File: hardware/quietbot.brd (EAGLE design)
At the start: 100 x 80 mm, 9 parts, among them IC2 REG1117

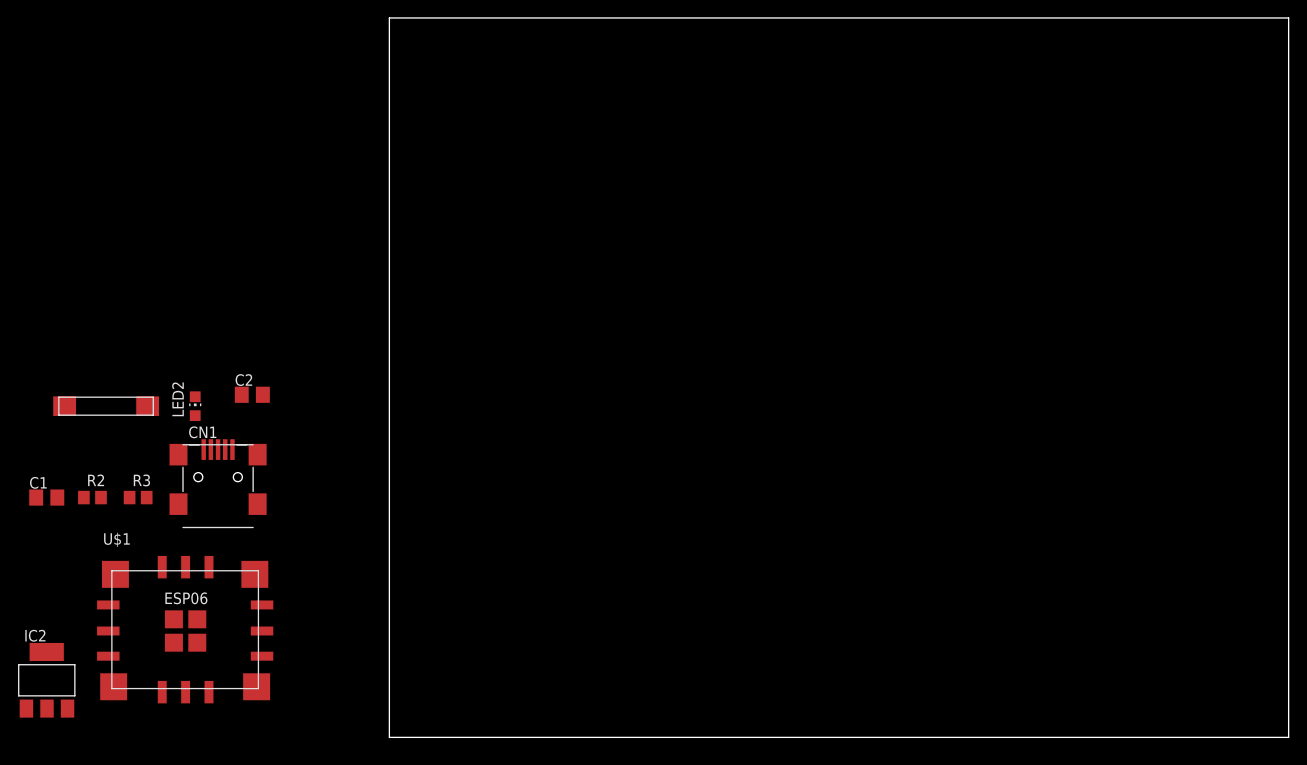
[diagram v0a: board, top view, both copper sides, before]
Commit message: board design
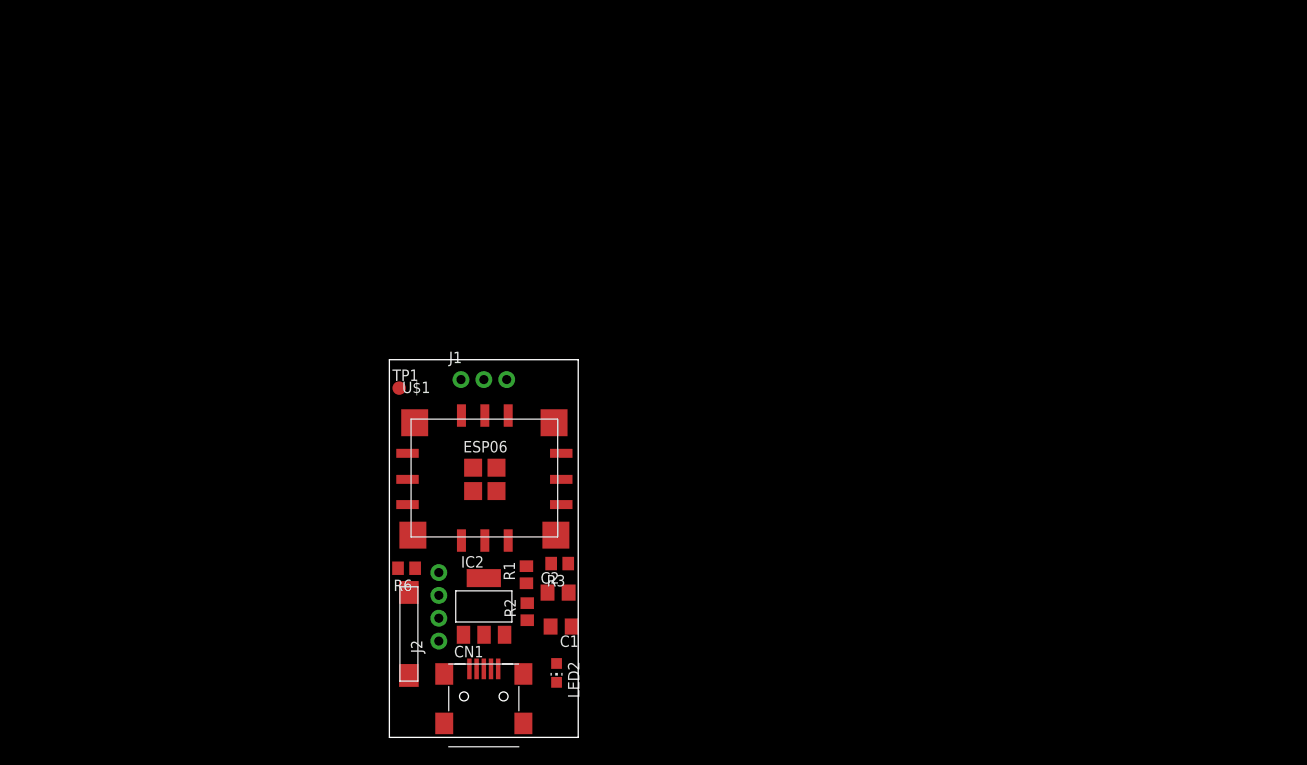
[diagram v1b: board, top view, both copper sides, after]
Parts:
- added J1: (no value), SparkFun-Connectors:1X03_NO_SILK
- added J2: (no value), SparkFun-Connectors:1X04_NO_SILK_ALL_ROUND
- added R1, R6: 10K, resistor:R0805
- added TP1: TPTP15R, testpad:TP15R
- moved C1 59.0 mm to (19.1, 12.3), turned to 180 degrees
- moved R2 50.0 mm to (15.3, 14.0), turned to 90 degrees
- moved LED2 49.9 mm to (18.6, 7.17), turned to 180 degrees
- moved IC2 49.3 mm to (10.5, 14.6)
- moved R3 47.5 mm to (18.9, 19.3), turned to 180 degrees
- moved U$2 42.5 mm to (2.17, 11.2), turned to 90 degrees
- moved C2 40.5 mm to (18.8, 16.1)
- moved CN1 38.3 mm to (10.5, 3.56)
- moved U$1 37.3 mm to (10.4, 28.3)
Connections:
- new net N$4: R6.2, TP1.TP, U$1.GPIO0
- new net N$5: R1.2, U$1.CH_PD
- new net RX: J2.2, U$1.RX
- new net SIG_PIXEL: J1.2, U$1.GPIO2
- new net TX: J2.3, U$1.TX
- net +3V3: now also J2.1, R1.1, R6.1; no longer U$1.CH_PD
- net +5V: now also J1.1
- net GND: now also J1.3, J2.4
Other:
- board size 100 x 80 mm -> 21 x 42 mm
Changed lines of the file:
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@@
 <setting verticaltext="up"/>
 </settings>
-<grid distance="0.05" unitdist="inch" unit="inch" style="lines" multiple="1" display="no" altdistance="0.025" altunitdist="inch" altunit="inch"/>
+<grid distance="1" unitdist="mm" unit="mm" style="lines" multiple="1" display="yes" altdistance="0.01" altunitdist="inch" altunit="inch"/>
 <layers>
 <layer number="1" name="Top" color="4" fill="1" visible="yes" active="yes"/>
@@
 <board>
 <plain>
-<wire x1="0" y1="0" x2="100" y2="0" width="0" layer="20"/>
-<wire x1="100" y1="0" x2="100" y2="80" width="0" layer="20"/>
-<wire x1="100" y1="80" x2="0" y2="80" width="0" layer="20"/>
-<wire x1="0" y1="80" x2="0" y2="0" width="0" layer="20"/>
+<wire x1="0" y1="0" x2="21" y2="0" width="0" layer="20"/>
+<wire x1="21" y1="0" x2="21" y2="42" width="0" layer="20"/>
+<wire x1="21" y1="42" x2="0" y2="42" width="0" layer="20"/>
+<wire x1="0" y1="42" x2="0" y2="0" width="0" layer="20"/>
 </plain>
 <attributes>
@@
 </autorouter>
 <elements>
-<element name="C1" library="rcl" package="R/2012-12R" value="10uF" x="-38.1" y="26.67"/>
-<element name="C2" library="rcl" package="R/2012-12R" value="10uF" x="-15.24" y="38.1"/>
-<element name="CN1" library="adafruit" package="USB-MINIB" value="" x="-19.05" y="27.94"/>
-<element name="IC2" library="burr-brown" package="SOT223" value="REG1117" x="-38.1" y="6.35">
-<attribute name="OC_FARNELL" value="1097566" x="-38.1" y="6.35" size="1.778" layer="27" display="off"/>
-<attribute name="MF" value="" x="-38.1" y="6.35" size="1.778" layer="27" display="off"/>
-<attribute name="MPN" value="LM1117 3v3" x="-38.1" y="6.35" size="1.778" layer="27" display="off"/>
-<attribute name="OC_NEWARK" value="14P6981" x="-38.1" y="6.35" size="1.778" layer="27" display="off"/>
+<element name="C1" library="rcl" package="R/2012-12R" value="10uF" x="19.1" y="12.33" rot="R180"/>
+<element name="C2" library="rcl" package="R/2012-12R" value="10uF" x="18.76" y="16.1"/>
+<element name="CN1" library="adafruit" package="USB-MINIB" value="" x="10.5" y="3.556"/>
+<element name="IC2" library="burr-brown" package="SOT223" value="REG1117" x="10.5" y="14.562">
+<attribute name="OC_FARNELL" value="1097566" x="10.5" y="14.562" size="1.778" layer="27" display="off"/>
+<attribute name="MF" value="" x="10.5" y="14.562" size="1.778" layer="27" display="off"/>
+<attribute name="MPN" value="LM1117 3v3" x="10.5" y="14.562" size="1.778" layer="27" display="off"/>
+<attribute name="OC_NEWARK" value="14P6981" x="10.5" y="14.562" size="1.778" layer="27" display="off"/>
 </element>
-<element name="LED2" library="led" package="CHIP-LED0805" value="GRN" x="-21.59" y="36.83"/>
-<element name="R2" library="resistor" package="R0805" value="1K" x="-33.02" y="26.67"/>
-<element name="R3" library="resistor" package="R0805" value="10K" x="-27.94" y="26.67"/>
-<element name="U$1" library="esp8266modules" package="ESP06" value="ESP06" x="-22.86" y="11.43"/>
-<element name="U$2" library="rainsun-ant" package="ANTENNA-CERAMIC" value="ANT" x="-31.75" y="36.83"/>
+<element name="LED2" library="led" package="CHIP-LED0805" value="GRN" x="18.59" y="7.17" rot="R180"/>
+<element name="R2" library="resistor" package="R0805" value="1K" x="15.33" y="13.98" rot="R90"/>
+<element name="R3" library="resistor" package="R0805" value="10K" x="18.94" y="19.33" rot="R180"/>
+<element name="U$1" library="esp8266modules" package="ESP06" value="ESP06" x="10.414" y="28.29"/>
+<element name="U$2" library="rainsun-ant" package="ANTENNA-CERAMIC" value="ANT" x="2.17" y="11.25" rot="R90"/>
+<element name="R6" library="resistor" package="R0805" value="10K" x="1.91" y="18.81" rot="R180"/>
+<element name="TP1" library="testpad" package="TP15R" value="TPTP15R" x="1.09" y="38.84">
+<attribute name="TP_SIGNAL_NAME" value="" x="1.09" y="38.84" size="1.778" layer="27" display="off"/>
+</element>
+<element name="R1" library="resistor" package="R0805" value="10K" x="15.24" y="18.09" rot="R90"/>
+<element name="J1" library="SparkFun-Connectors" package="1X03_NO_SILK" value="" x="7.964" y="39.79"/>
+<element name="J2" library="SparkFun-Connectors" package="1X04_NO_SILK_ALL_ROUND" value="" x="5.498" y="10.71" rot="R90">
+<attribute name="PROD_ID" value="CONN-09696" x="5.498" y="10.71" size="1.778" layer="27" rot="R90" display="off"/>
+</element>
 </elements>
 <signals>
@@
 <contactref element="C1" pad="+"/>
 <contactref element="CN1" pad="VBUS"/>
-<wire x1="-36.925" y1="26.67" x2="-35.7886" y2="3.2004" width="0" layer="19" extent="1-1"/>
-<wire x1="-20.65" y1="32.004" x2="-36.925" y2="26.67" width="0" layer="19" extent="1-1"/>
+<contactref element="J1" pad="1"/>
+<wire x1="12.8114" y1="11.4124" x2="7.964" y2="39.79" width="0" layer="19" extent="1-1"/>
+<wire x1="17.925" y1="12.33" x2="12.8114" y2="11.4124" width="0" layer="19" extent="1-1"/>
+<wire x1="8.9" y1="7.62" x2="17.925" y2="12.33" width="0" layer="19" extent="1-1"/>
 </signal>
 <signal name="GND">
@@
 <contactref element="R2" pad="1"/>
 <contactref element="R3" pad="1"/>
+<contactref element="J1" pad="3"/>
+<contactref element="J2" pad="4"/>
 <contactref element="U$1" pad="GND6"/>
-<wire x1="-21.36" y1="10.53" x2="-40.3606" y2="3.2004" width="0" layer="19" extent="1-1"/>
-<wire x1="-28.89" y1="26.67" x2="-21.36" y2="10.53" width="0" layer="19" extent="1-1"/>
-<wire x1="-33.97" y1="26.67" x2="-28.89" y2="26.67" width="0" layer="19" extent="1-1"/>
-<wire x1="-39.275" y1="26.67" x2="-33.97" y2="26.67" width="0" layer="19" extent="1-1"/>
-<wire x1="-17.45" y1="32.004" x2="-28.89" y2="26.67" width="0" layer="19" extent="1-1"/>
-<wire x1="-16.415" y1="38.1" x2="-17.45" y2="32.004" width="0" layer="19" extent="1-1"/>
+<wire x1="13.044" y1="39.79" x2="5.498" y2="18.33" width="0" layer="19" extent="1-1"/>
+<wire x1="8.2394" y1="11.4124" x2="13.044" y2="39.79" width="0" layer="19" extent="1-1"/>
+<wire x1="11.914" y1="27.39" x2="8.2394" y2="11.4124" width="0" layer="19" extent="1-1"/>
+<wire x1="19.89" y1="19.33" x2="11.914" y2="27.39" width="0" layer="19" extent="1-1"/>
+<wire x1="15.33" y1="13.03" x2="19.89" y2="19.33" width="0" layer="19" extent="1-1"/>
+<wire x1="20.275" y1="12.33" x2="15.33" y2="13.03" width="0" layer="19" extent="1-1"/>
+<wire x1="12.1" y1="7.62" x2="19.89" y2="19.33" width="0" layer="19" extent="1-1"/>
+<wire x1="17.585" y1="16.1" x2="12.1" y2="7.62" width="0" layer="19" extent="1-1"/>
 </signal>
 <signal name="+3V3">
@@
 <contactref element="C2" pad="+"/>
 <contactref element="U$1" pad="VCC"/>
-<contactref element="U$1" pad="CH_PD"/>
 <contactref element="LED2" pad="A"/>
-<wire x1="-31.26" y1="9.03" x2="-38.0746" y2="3.2004" width="0" layer="19" extent="1-1"/>
-<wire x1="-31.26" y1="11.83" x2="-31.26" y2="9.03" width="0" layer="19" extent="1-1"/>
-<wire x1="-21.59" y1="35.78" x2="-31.26" y2="11.83" width="0" layer="19" extent="1-1"/>
-<wire x1="-14.065" y1="38.1" x2="-21.59" y2="35.78" width="0" layer="19" extent="1-1"/>
+<contactref element="R6" pad="1"/>
+<contactref element="R1" pad="1"/>
+<contactref element="J2" pad="1"/>
+<wire x1="15.24" y1="17.14" x2="5.498" y2="10.71" width="0" layer="19" extent="1-1"/>
+<wire x1="2.86" y1="18.81" x2="15.24" y2="17.14" width="0" layer="19" extent="1-1"/>
+<wire x1="10.5254" y1="11.4124" x2="2.86" y2="18.81" width="0" layer="19" extent="1-1"/>
+<wire x1="2.014" y1="28.69" x2="10.5254" y2="11.4124" width="0" layer="19" extent="1-1"/>
+<wire x1="18.59" y1="8.22" x2="2.014" y2="28.69" width="0" layer="19" extent="1-1"/>
+<wire x1="19.935" y1="16.1" x2="18.59" y2="8.22" width="0" layer="19" extent="1-1"/>
 </signal>
 <signal name="N$2">
 <contactref element="R2" pad="2"/>
 <contactref element="LED2" pad="C"/>
-<wire x1="-32.07" y1="26.67" x2="-21.59" y2="37.88" width="0" layer="19" extent="1-1"/>
+<wire x1="15.33" y1="14.93" x2="18.59" y2="6.12" width="0" layer="19" extent="1-1"/>
 </signal>
 <signal name="N$1">
 <contactref element="U$1" pad="GPIO15"/>
 <contactref element="R3" pad="2"/>
-<wire x1="-26.99" y1="26.67" x2="-14.16" y2="9.03" width="0" layer="19" extent="1-1"/>
+<wire x1="17.99" y1="19.33" x2="19.114" y2="25.89" width="0" layer="19" extent="1-1"/>
 </signal>
 <signal name="N$3">
 <contactref element="U$2" pad="FEED"/>
 <contactref element="U$1" pad="ANT"/>
-<wire x1="-26.885" y1="36.83" x2="-31.26" y2="14.73" width="0" layer="19" extent="1-1"/>
+<wire x1="2.17" y1="16.115" x2="2.014" y2="31.59" width="0" layer="19" extent="1-1"/>
+</signal>
+<signal name="N$4">
+<contactref element="U$1" pad="GPIO0"/>
+<contactref element="R6" pad="2"/>
+<contactref element="TP1" pad="TP"/>
+<wire x1="0.96" y1="18.81" x2="1.09" y2="38.84" width="0" layer="19" extent="1-1"/>
+<wire x1="19.114" y1="31.59" x2="0.96" y2="18.81" width="0" layer="19" extent="1-1"/>
+</signal>
+<signal name="N$5">
+<contactref element="R1" pad="2"/>
+<contactref element="U$1" pad="CH_PD"/>
+<wire x1="2.014" y1="25.89" x2="15.24" y2="19.04" width="0" layer="19" extent="1-1"/>
+</signal>
+<signal name="RX">
+<contactref element="U$1" pad="RX"/>
+<contactref element="J2" pad="2"/>
+<wire x1="13.214" y1="35.79" x2="5.498" y2="13.25" width="0" layer="19" extent="1-1"/>
+</signal>
+<signal name="TX">
+<contactref element="U$1" pad="TX"/>
+<contactref element="J2" pad="3"/>
+<wire x1="10.614" y1="35.79" x2="5.498" y2="15.79" width="0" layer="19" extent="1-1"/>
+</signal>
+<signal name="SIG_PIXEL">
+<contactref element="U$1" pad="GPIO2"/>
+<contactref element="J1" pad="2"/>
+<wire x1="19.114" y1="28.69" x2="10.504" y2="39.79" width="0" layer="19" extent="1-1"/>
 </signal>
 </signals>
